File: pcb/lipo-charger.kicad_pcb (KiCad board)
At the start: 2 copper layers, 48 x 48 mm, 37 parts, among them J101 Barrel_Jack, J102 Conn_01x04, J103 Conn_01x03, J104 Conn_01x03, J201 Conn_01x02, J202 Conn_01x02, P101 Polarity, P102 Outline, P103 OSHW, Q201 Q_NMOS_GSD, U101 LM317L_TO92, U201 MP2359, U202 LM358, U203 MAX4377, U204 LM358

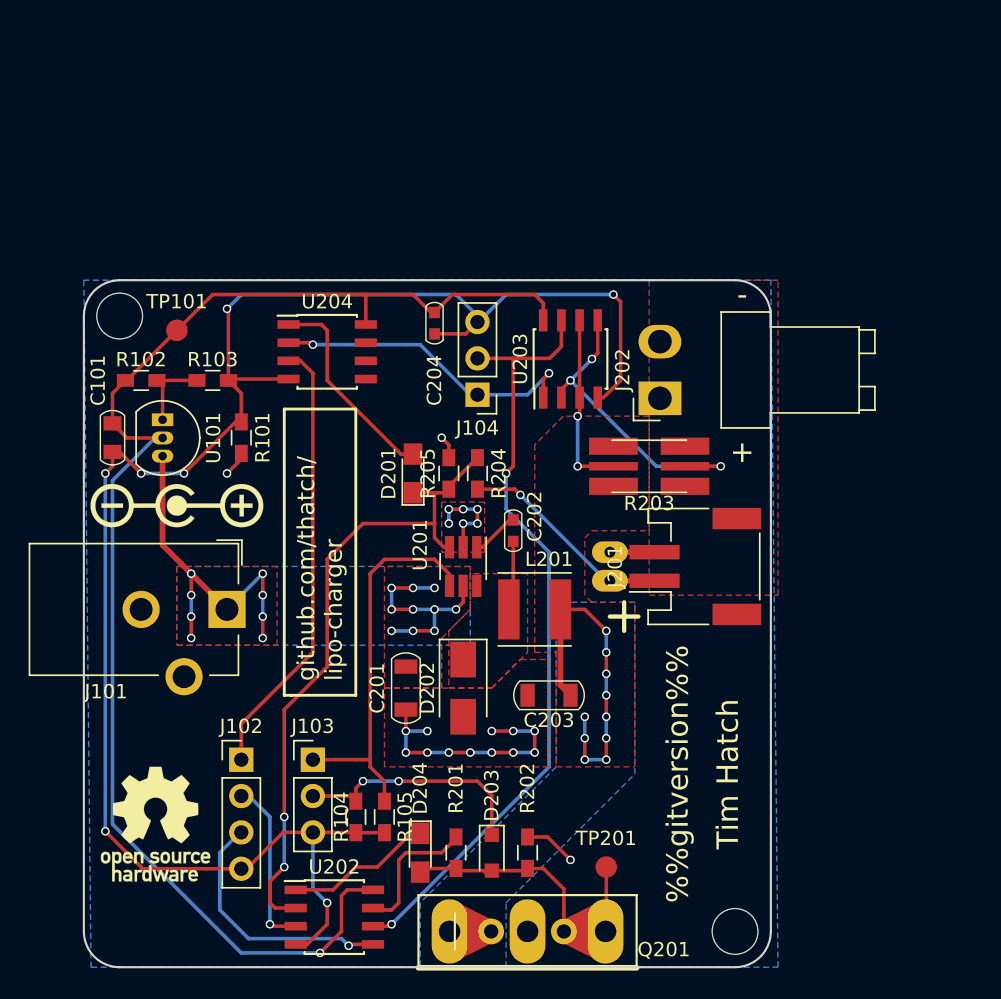
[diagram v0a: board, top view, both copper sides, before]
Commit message: Massive rework, fully routed
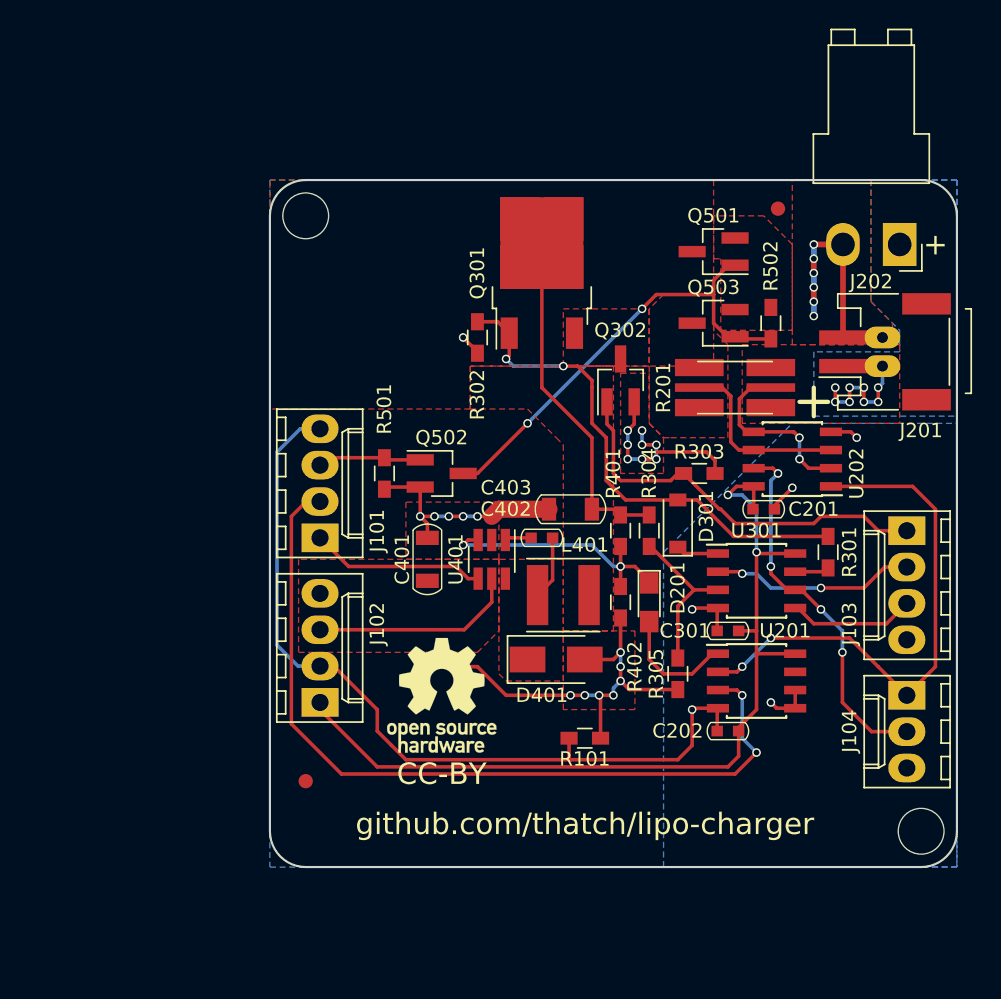
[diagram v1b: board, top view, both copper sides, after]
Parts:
- removed C101: 1u, Capacitors_SMD_Round:C_0805
- removed C203: 22u, Capacitors_SMD_Round:C_1206
- removed C204: 0.1u, Capacitors_SMD_Round:C_0603
- removed D202: B230A, Diodes_SMD:D_SMA
- removed D203: B5819, Diodes_SMD:D_SOD-323_HandSoldering
- removed D204: LED, LEDs:LED_0805_HandSoldering
- removed L201: 4.7uH, Inductors_SMD:L_Taiyo-Yuden_NR-50xx
- removed Q201: Q_NMOS_GSD, TO_Combo_Packages:TO_220_247
- removed R102: 330R, Resistors_SMD:R_0603_HandSoldering
- removed R103: 2k, Resistors_SMD:R_0603_HandSoldering
- removed R104, R105: 10k, Resistors_SMD:R_0603_HandSoldering
- removed R202: 100k, Resistors_SMD:R_0603_HandSoldering
- removed R203: 0R025, Sense_Resistors:R_2512_AD_Optimized
- removed R204: 107k, Resistors_SMD:R_0603_HandSoldering
- removed R205: 25.5k, Resistors_SMD:R_0603_HandSoldering
- removed TP101, TP201: TEST, Measurement_Points:Measurement_Point_Round-SMD-Pad_Small
- removed U101: LM317L_TO92, TO_SOT_Packages_THT:TO-92_Inline_Narrow_Oval
- removed U203: MAX4377, Housings_SOIC:SOIC-8_3.9x4.9mm_Pitch1.27mm
- removed U204: LM358, Housings_SOIC:SOIC-8_3.9x4.9mm_Pitch1.27mm
- added C301: 0.1u, Capacitors_SMD_Round:C_0603, F.Cu at (159.5, 109.5)
- added C401: 10u, Capacitors_SMD_Round:C_1206, F.Cu at (138.5, 104.5)
- added C402: 10n, Capacitors_SMD_Round:C_0603, F.Cu at (146.5, 103.0)
- added C403: 22u, Capacitors_SMD_Round:C_1206, F.Cu at (148.5, 101.0)
- added D301: D_Schottky, Diodes_SMD:D_SOD-123, F.Cu at (156.0, 102.0)
- added D401: B230A, Diodes_SMD:D_SMA, F.Cu at (147.5, 111.5)
- added L401: 4.7uH, Inductors_SMD:L_Taiyo-Yuden_NR-50xx, F.Cu at (148.0, 107.0)
- added P104: Fid, Fiducials:Fiducial_1mm_Dia_2.54mm_Outer_CopperTop, F.Cu at (130.0, 120.0)
- added Q301: Q_NMOS_GDS, TO_SOT_Packages_SMD:TO-252-2, F.Cu at (146.5, 84.5)
- added Q302: Q_NMOS_GSD, TO_SOT_Packages_SMD:SOT-23_Handsoldering, F.Cu at (152.0, 92.0)
- added Q501: Q_PMOS_GSD, TO_SOT_Packages_SMD:SOT-23_Handsoldering, F.Cu at (158.5, 83.0)
- added Q502: Q_NMOS_GSD, TO_SOT_Packages_SMD:SOT-23_Handsoldering, F.Cu at (139.5, 98.5)
- added Q503: Q_PMOS_GSD, TO_SOT_Packages_SMD:SOT-23_Handsoldering, F.Cu at (158.5, 88.0)
- added R301: 100R, Resistors_SMD:R_0603_HandSoldering, F.Cu at (166.5, 104.0)
- added R302: 100k, Resistors_SMD:R_0603_HandSoldering, F.Cu at (142.0, 89.0)
- added R303: 100k, Resistors_SMD:R_0603_HandSoldering, F.Cu at (157.5, 98.5)
- added R304: 100k, Resistors_SMD:R_0603_HandSoldering, F.Cu at (154.0, 102.5)
- added R305: 100k, Resistors_SMD:R_0603_HandSoldering, F.Cu at (156.0, 112.5)
- added R401: 107k, Resistors_SMD:R_0603_HandSoldering, F.Cu at (152.0, 102.5)
- added R402: 25.5k, Resistors_SMD:R_0603_HandSoldering, F.Cu at (152.0, 107.5)
- added R501: 100k, Resistors_SMD:R_0603_HandSoldering, F.Cu at (135.5, 98.5)
- added R502: 100k, Resistors_SMD:R_0603_HandSoldering, F.Cu at (162.5, 88.0)
- added U301: LM358, Housings_SOIC:SOIC-8_3.9x4.9mm_Pitch1.27mm, F.Cu at (161.5, 106.0)
- added U401: MP2359, TO_SOT_Packages_SMD:SOT-23-6_Handsoldering, F.Cu at (143.0, 104.5)
- C201: value 10u -> 0.1u; footprint Capacitors_SMD_Round:C_1206 -> Capacitors_SMD_Round:C_0603
- C202: value 10n -> 0.1u
- J101: value Barrel_Jack -> Conn_01x04; footprint Connectors:Barrel_Jack_CUI_PJ-102AH -> Connectors_Molex:Molex_KK-6410-04_04x2.54mm_Straight
- J102: footprint Pin_Headers:Pin_Header_Straight_1x04_Pitch2.54mm -> Connectors_Molex:Molex_KK-6410-04_04x2.54mm_Straight
- J103: value Conn_01x03 -> Conn_01x04; footprint Pin_Headers:Pin_Header_Straight_1x03_Pitch2.54mm -> Connectors_Molex:Molex_KK-6410-04_04x2.54mm_Straight
- J104: footprint Pin_Headers:Pin_Header_Straight_1x03_Pitch2.54mm -> Connectors_Molex:Molex_KK-6410-03_03x2.54mm_Straight
- P101: value Polarity -> Fid; footprint Polarity_Symbols:Polarity_Center_Positive_3mm_SilkScreen -> Fiducials:Fiducial_1mm_Dia_2.54mm_Outer_CopperTop
- R101: value 0R -> 100R
- R201: value 10k -> 0R025; footprint Resistors_SMD:R_0603_HandSoldering -> Sense_Resistors:R_2512_AD_Optimized
- U201: value MP2359 -> LM358; footprint TO_SOT_Packages_SMD:SOT-23-6_Handsoldering -> Housings_SOIC:SOIC-8_3.9x4.9mm_Pitch1.27mm
- U202: value LM358 -> MAX4377
- moved P101 46.8 mm to (163.0, 80.0)
- moved U202 45.3 mm to (164.0, 97.5), turned to 180 degrees
- moved J103 44.5 mm to (172.0, 102.5), turned to 270 degrees
- moved R201 37.9 mm to (160.0, 92.5), turned to 180 degrees
- moved J104 36.6 mm to (172.0, 114.0), turned to 270 degrees
- moved R101 31.9 mm to (149.5, 117.0), turned to 180 degrees
- moved C201 28.0 mm to (162.0, 101.0), turned to 0 degrees
- moved U201 22.0 mm to (161.5, 113.0), turned to 0 degrees
- moved P103 21.9 mm to (139.5, 114.0)
- moved C202 20.5 mm to (159.5, 116.5), turned to 180 degrees
- moved J201 20.0 mm to (170.5, 90.0)
- moved J202 19.9 mm to (171.5, 82.5), turned to 180 degrees
- moved D201 18.8 mm to (154.0, 107.5), turned to 270 degrees
- moved P102 14.8 mm to (127.5, 78.0)
- moved J101 8.20 mm to (131.0, 103.0), turned to 90 degrees
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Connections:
- C201 pad 1: /charger/VIN -> +9VA
- C201 pad 2: GND -> GNDA
- C202 pad 1: Net-(C202-Pad1) -> +9VA
- C202 pad 2: /charger/Vsw -> GNDA
- D201 pad 1: Net-(D201-Pad1) -> /charger/buck/FB
- J101 pad 1: /charger/VIN -> /charger/CHG_EN
- J101 pad 2: GND -> /charger/CHG_AREF
- J101 pad 3: GND -> /charger/MASTER_EN
- J102 pad 1: /charger/CHG_AREF -> +9VA
- J102 pad 2: /charger/LOAD_VREF -> GNDA
- J102 pad 3: /charger/LOAD_AREF -> /charger/VIN
- J102 pad 4: GNDA -> /charger/GNDIN
- J103 pad 1: /charger/CHG_EN -> /charger/LOAD_EN
- J103 pad 2: /charger/LOAD_EN -> /charger/LOAD_VREF
- J103 pad 3: GNDA -> /charger/LOAD_AREF
- J201 pad 2: GND -> /charger/GNDIN
- J202 pad 2: GND -> /charger/GNDIN
- R101 pad 1: GND -> /charger/GNDIN
- R201 pad 1: Net-(R201-Pad1) -> /charger/BATPLUS
- R201 pad 2: Net-(D203-Pad2) -> Net-(R201-Pad2)
- U201 pad 1: Net-(C202-Pad1) -> Net-(D201-Pad2)
- U201 pad 2: GND -> /charger/OUT1
- U201 pad 3: Net-(D201-Pad1) -> /charger/CHG_AREF
- U201 pad 4: /charger/CHG_EN -> GNDA
- U201 pad 5: /charger/VIN -> GNDA
- U201 pad 6: /charger/Vsw -> GNDA
- U202 pad 1: Net-(D204-Pad1) -> /charger/OUT1
- U202 pad 2: Net-(D201-Pad1) -> Net-(R201-Pad2)
- U202 pad 3: /charger/LOAD_VREF -> Net-(R201-Pad3)
- U202 pad 5: /charger/LOAD_AREF -> Net-(R201-Pad2)
- U202 pad 6: /charger/OUT2 -> Net-(R201-Pad3)
- U202 pad 7: Net-(R201-Pad1) -> /charger/OUT2
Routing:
- net /charger/GNDIN: track 0.00 -> 74.9 mm, vias 0 -> 27
- net GNDA: track 123.0 -> 69.0 mm, vias 7 -> 5
- net Net-(D201-Pad1): track 46.2 -> 0.00 mm, vias 2 -> 0
- net Net-(D301-Pad2): track 0.00 -> 36.0 mm, vias 0 -> 2
- net +9VA: track 97.7 -> 62.3 mm, vias 1 -> 2
- net GND: track 34.9 -> 0.00 mm, vias 21 -> 0
- net Net-(Q501-Pad1): track 0.00 -> 32.1 mm, vias 0 -> 2
- net /charger/VIN: track 44.0 -> 14.4 mm, vias 18 -> 0
- net /charger/OUT2: track 55.0 -> 26.1 mm, vias 2 -> 4
- net /charger/CHG_AREF: track 31.1 -> 58.8 mm, vias 0 -> 2
- net /charger/Ind_out: track 26.5 -> 0.00 mm, vias 10 -> 0
- net /charger/output_disconnect/LOAD_CHARGE: track 0.00 -> 24.2 mm
- net Net-(R203-Pad2): track 22.4 -> 0.00 mm, vias 3 -> 0
- net Net-(D203-Pad2): track 21.7 -> 0.00 mm
- net /charger/buck/FB: track 0.00 -> 18.2 mm, vias 0 -> 2
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- added copper zone on B.Cu, net /charger/BATPLUS
- added copper zone on B.Cu, net /charger/GNDIN
- added copper zone on F.Cu, net /charger/GNDIN
- added copper zone on F.Cu, net /charger/buck/Vsw
- added copper zone on F.Cu, net /charger/output_disconnect/BATT
- added copper zone on F.Cu, net /charger/output_disconnect/LOAD_CHARGE
- added copper zone on B.Cu, net GNDA
- added copper zone on F.Cu, net Net-(Q301-Pad3)
- added copper zone on F.Cu, net Net-(Q501-Pad2)
- removed copper zone on B.Cu, net /charger/Ind_out
- removed copper zone on F.Cu, net /charger/Ind_out
- removed copper zone on B.Cu, net /charger/VIN
- removed copper zone on F.Cu, net /charger/Vsw
- removed copper zone on B.Cu, net GND
- removed copper zone on F.Cu, net GND
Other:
- board text added: "CC-BY"
- board text added: "GNDA MASTER_EN CHG_AREF CHG_EN"
- board text added: "LOAD_EN LOAD_VREF LOAD_AREF GNDA"
- board text added: "OUT1 OUT2 GNDA"
- board text added: "Power GND Power VIN GNDA +9VA"
- board text added: "github.com/thatch/lipo-charger"
- board text removed: "%%gitversion%%"
- board text removed: "-"
- board text removed: "Tim Hatch"
- board text removed: "github.com/thatch/ lipo-charger"
